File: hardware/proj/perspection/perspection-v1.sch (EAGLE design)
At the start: 187 parts, among them J1 MICRO-USB-10118192-0001LF, Q1 CSD18533Q5A, Q2 CSD18533Q5A, Q3 CSD18533Q5A, Q4 CSD18533Q5A, Q5 CSD18533Q5A, Q6 CSD18533Q5A, U1 ATUM, U10 DRV8301DCAR, U11 OPA2374AIDCNR, U2 FT232RQ, U3 TPS79933DDCR, U4 MCP73831T-2ACI/OT, U5 TMS320F28069MPZT, U6 DRV8801PWPR, U7 DRV8801PWPR, U8 DRV8801PWPR, U9 DRV8801PWPR

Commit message: parts and LED circuit and shit
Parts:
- added D6: LED-PWR-XLAMP_MX3, perspection:LED-PWR-XLAMP_MX3
- added Q7: NMOS-CSD18533Q5A, perspection:NMOS-CSD18533Q5A
- added R79: (no value), perspection:R0805
- added R80: (no value), perspection:R0402
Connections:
- new net N$59: D6.CATHODE, Q7.D
- new net N$60: Q7.S, R79.2
- new net N$61: Q7.G, R80.1
- net GND: now also R79.1
- net VBAT: now also D6.ANODE
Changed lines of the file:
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@@
 <setting verticaltext="up"/>
 </settings>
-<grid distance="0.1" unitdist="inch" unit="inch" style="lines" multiple="1" display="yes" altdistance="0.01" altunitdist="inch" altunit="inch"/>
+<grid distance="0.1" unitdist="inch" unit="inch" style="lines" multiple="1" display="no" altdistance="0.01" altunitdist="inch" altunit="inch"/>
 <layers>
 <layer number="1" name="Top" color="4" fill="1" visible="no" active="no"/>
@@
 <part name="+3V18" library="perspection" deviceset="+3V3" device=""/>
 <part name="GND63" library="perspection" deviceset="GND" device=""/>
+<part name="P+15" library="perspection" deviceset="VBAT" device=""/>
+<part name="FRAME7" library="perspection" deviceset="A3L-LOC" device=""/>
+<part name="Q7" library="perspection" deviceset="NMOS" device="-CSD18533Q5A"/>
+<part name="D6" library="perspection" deviceset="LED-PWR" device="-XLAMP_MX3"/>
+<part name="R79" library="perspection" deviceset="R" device="0805"/>
+<part name="GND64" library="perspection" deviceset="GND" device=""/>
+<part name="R80" library="perspection" deviceset="R" device="0402"/>
 </parts>
 <sheets>
@@
 </segment>
 </net>
+</nets>
+</sheet>
+<sheet>
+<plain>
+</plain>
+<instances>
+<instance part="P+15" gate="G$1" x="66.04" y="101.6"/>
+<instance part="FRAME7" gate="G$1" x="0" y="0"/>
+<instance part="Q7" gate="G$1" x="63.5" y="83.82"/>
+<instance part="D6" gate="G$1" x="66.04" y="93.98" rot="R270"/>
+<instance part="R79" gate="G$1" x="66.04" y="63.5" rot="R90"/>
+<instance part="GND64" gate="1" x="66.04" y="50.8"/>
+<instance part="R80" gate="G$1" x="53.34" y="81.28" rot="R180"/>
+</instances>
+<busses>
+</busses>
+<nets>
+<net name="VBAT" class="0">
+<segment>
+<pinref part="D6" gate="G$1" pin="ANODE"/>
+<pinref part="P+15" gate="G$1" pin="VBAT"/>
+<wire x1="66.04" y1="99.06" x2="66.04" y2="101.6" width="0.1524" layer="91"/>
+</segment>
+</net>
+<net name="N$59" class="0">
+<segment>
+<pinref part="D6" gate="G$1" pin="CATHODE"/>
+<pinref part="Q7" gate="G$1" pin="D"/>
+<wire x1="66.04" y1="88.9" x2="66.04" y2="91.44" width="0.1524" layer="91"/>
+</segment>
+</net>
+<net name="N$60" class="0">
+<segment>
+<pinref part="Q7" gate="G$1" pin="S"/>
+<pinref part="R79" gate="G$1" pin="2"/>
+<wire x1="66.04" y1="68.58" x2="66.04" y2="78.74" width="0.1524" layer="91"/>
+</segment>
+</net>
+<net name="GND" class="0">
+<segment>
+<pinref part="R79" gate="G$1" pin="1"/>
+<pinref part="GND64" gate="1" pin="GND"/>
+<wire x1="66.04" y1="53.34" x2="66.04" y2="58.42" width="0.1524" layer="91"/>
+</segment>
+</net>
+<net name="N$61" class="0">
+<segment>
+<pinref part="Q7" gate="G$1" pin="G"/>
+<pinref part="R80" gate="G$1" pin="1"/>
+<wire x1="58.42" y1="81.28" x2="60.96" y2="81.28" width="0.1524" layer="91"/>
+</segment>
+</net>

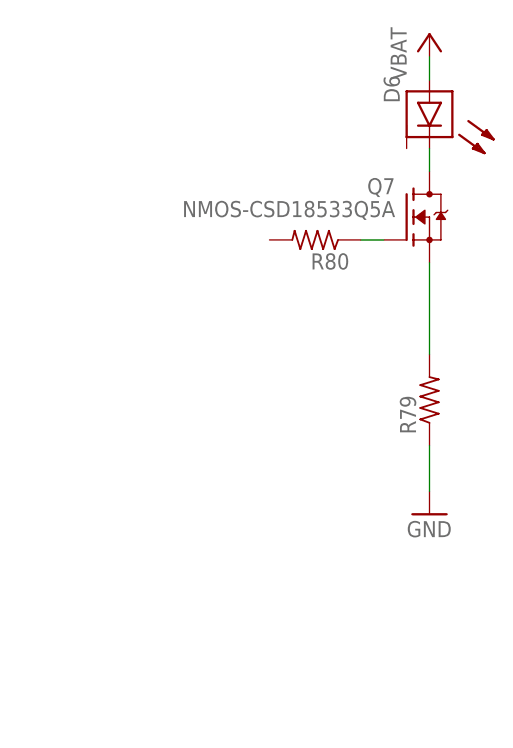
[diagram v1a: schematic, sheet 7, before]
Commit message: started led thing
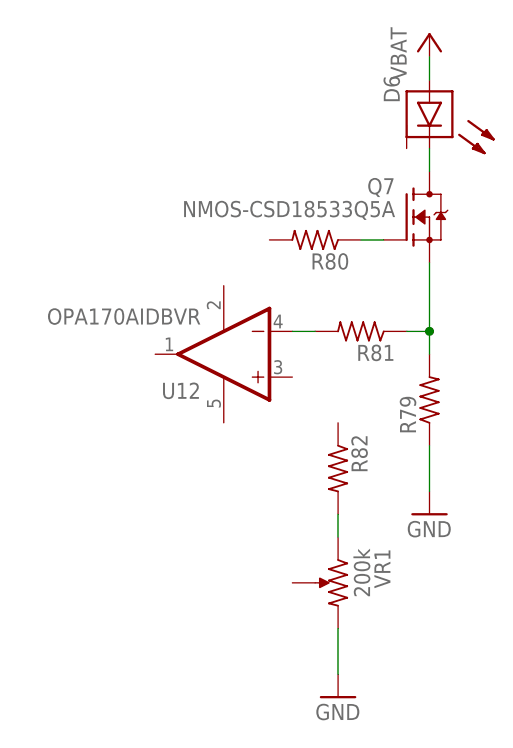
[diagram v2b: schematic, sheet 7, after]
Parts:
- added R81, R82: (no value), perspection:R0402
- added U12: OPA170AIDBVR, perspection:OPA170AIDBVR
- added VR1: 200k, perspection:R-TRIM-ST4ETA204
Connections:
- new net N$62: R81.2, U12.-IN
- new net N$63: R82.2, VR1.1
- net GND: now also VR1.2
- net N$60: now also R81.1
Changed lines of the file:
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@@
 <part name="GND64" library="perspection" deviceset="GND" device=""/>
 <part name="R80" library="perspection" deviceset="R" device="0402"/>
+<part name="U12" library="perspection" deviceset="OPA170" device="AIDBVR"/>
+<part name="R81" library="perspection" deviceset="R" device="0402"/>
+<part name="R82" library="perspection" deviceset="R" device="0402"/>
+<part name="VR1" library="perspection" deviceset="R-TRIM" device="-ST4ETA204" value="200k"/>
+<part name="GND65" library="perspection" deviceset="GND" device=""/>
 </parts>
 <sheets>
@@
 <instance part="GND64" gate="1" x="66.04" y="50.8"/>
 <instance part="R80" gate="G$1" x="53.34" y="81.28" rot="R180"/>
+<instance part="U12" gate="G$1" x="43.18" y="68.58" rot="R180"/>
+<instance part="R81" gate="G$1" x="58.42" y="71.12" rot="R180"/>
+<instance part="R82" gate="G$1" x="55.88" y="55.88" rot="R270"/>
+<instance part="VR1" gate="G$1" x="55.88" y="43.18" rot="R270"/>
+<instance part="GND65" gate="1" x="55.88" y="30.48"/>
 </instances>
 <busses>
@@
 </segment>
 </net>
-<net name="N$60" class="0">
-<segment>
-<pinref part="Q7" gate="G$1" pin="S"/>
-<pinref part="R79" gate="G$1" pin="2"/>
-<wire x1="66.04" y1="68.58" x2="66.04" y2="78.74" width="0.1524" layer="91"/>
-</segment>
-</net>
 <net name="GND" class="0">
 <segment>
@@
 <wire x1="66.04" y1="53.34" x2="66.04" y2="58.42" width="0.1524" layer="91"/>
 </segment>
+<segment>
+<pinref part="VR1" gate="G$1" pin="2"/>
+<pinref part="GND65" gate="1" pin="GND"/>
+<wire x1="55.88" y1="33.02" x2="55.88" y2="38.1" width="0.1524" layer="91"/>
+</segment>
 </net>
 <net name="N$61" class="0">
@@
 </segment>
 </net>
+<net name="N$62" class="0">
+<segment>
+<pinref part="R81" gate="G$1" pin="2"/>
+<pinref part="U12" gate="G$1" pin="-IN"/>
+<wire x1="50.8" y1="71.12" x2="53.34" y2="71.12" width="0.1524" layer="91"/>
+</segment>
+</net>
+<net name="N$60" class="0">
+<segment>
+<pinref part="Q7" gate="G$1" pin="S"/>
+<pinref part="R79" gate="G$1" pin="2"/>
+<wire x1="66.04" y1="78.74" x2="66.04" y2="71.12" width="0.1524" layer="91"/>
+<pinref part="R81" gate="G$1" pin="1"/>
+<wire x1="66.04" y1="71.12" x2="66.04" y2="68.58" width="0.1524" layer="91"/>
+<wire x1="63.5" y1="71.12" x2="66.04" y2="71.12" width="0.1524" layer="91"/>
+<junction x="66.04" y="71.12"/>
+</segment>
+</net>
+<net name="N$63" class="0">
+<segment>
+<pinref part="R82" gate="G$1" pin="2"/>
+<pinref part="VR1" gate="G$1" pin="1"/>
+<wire x1="55.88" y1="48.26" x2="55.88" y2="50.8" width="0.1524" layer="91"/>
+</segment>
+</net>
